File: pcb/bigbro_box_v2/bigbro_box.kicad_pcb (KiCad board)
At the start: 2 copper layers, 100 x 58 mm, 44 parts, among them J1 Current Sense, J2 Display, J3 Mains, J4 Debug, J5 RFID, J6 Relay, J7 Ext, K1 G5LE-1, Q1 MMBT3904, Q2 MMBT3904, Q3 BSS138, Q4 MMBT3906, SW1 Card switch, U1 ESP32-WROOM-32, U2 AP1117-33, U3 4011, U4 4011, U5 RDM6300

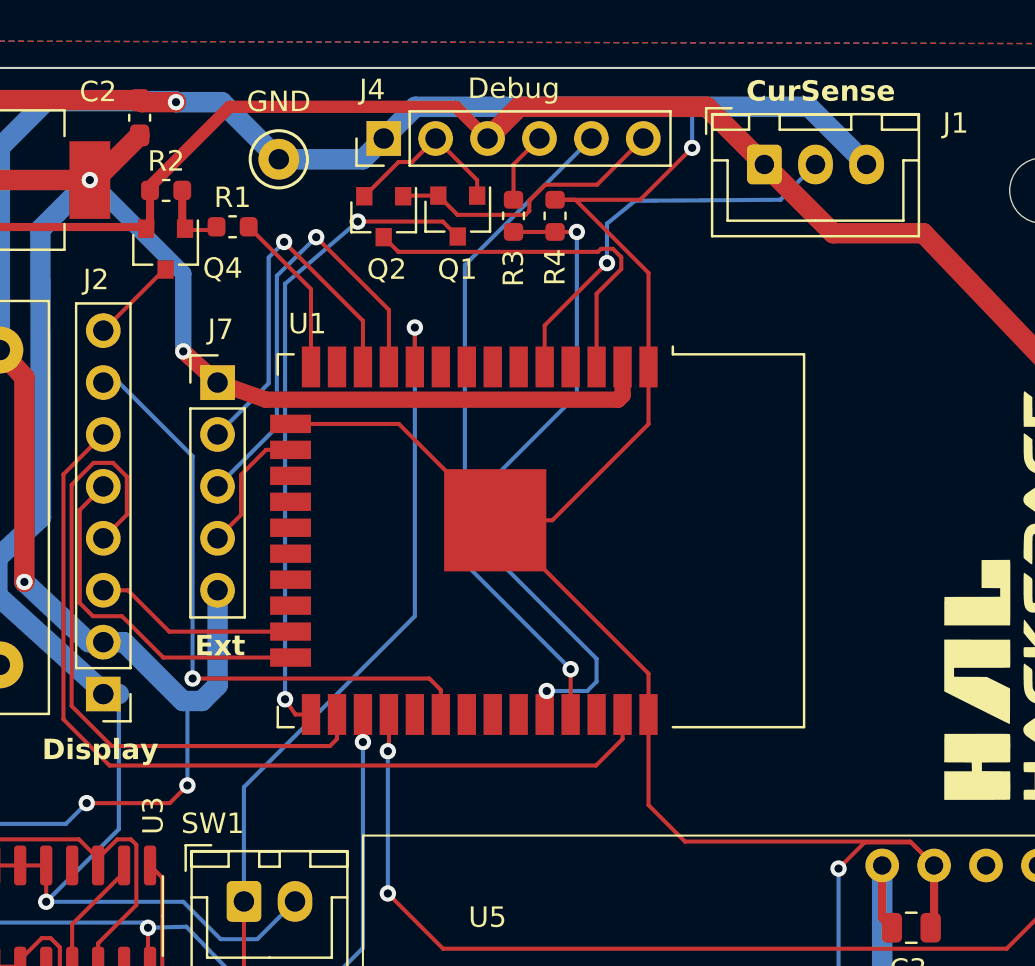
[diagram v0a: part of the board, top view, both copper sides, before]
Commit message: Order.
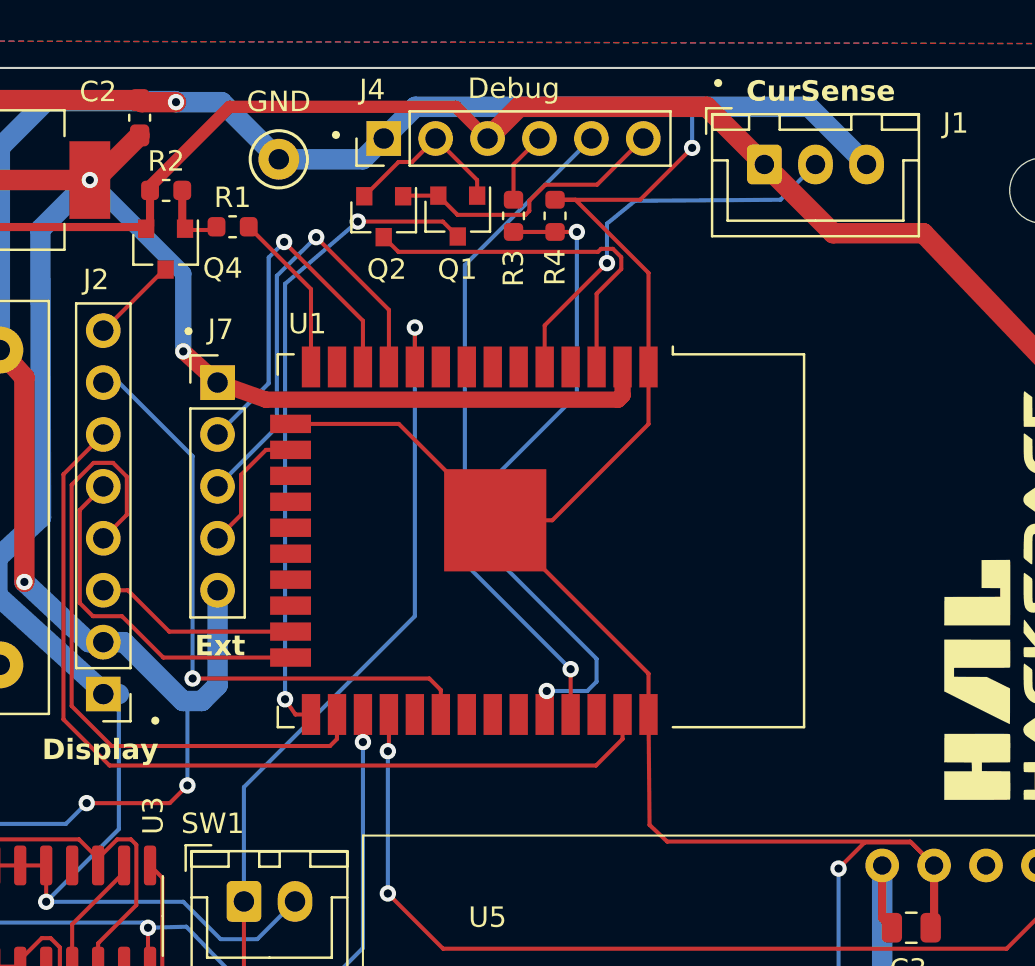
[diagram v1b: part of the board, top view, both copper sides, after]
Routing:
- net GND: track 282.3 -> 282.8 mm
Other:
- board text added: "•"
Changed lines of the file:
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@@
     (pad "1" thru_hole circle (at 0 0) (size 2 2) (drill 1) (layers "*.Cu" "*.Mask")
       (net 2 "GND") (pinfunction "1") (pintype "passive"))
-    (model "${KICAD6_3DMODEL_DIR}/TestPoint.3dshapes/TestPoint_Keystone_5000-5004_Miniature.wrl"
+    (model "${KIPRJMOD}/lib/3D/TestPoint_Loop_D2.60mm_Drill0.9mm_Beaded.step"
       (offset (xyz 0 0 0))
       (scale (xyz 1 1 1))
@@
     (effects (font (size 1 1) (thickness 0.18) bold) (justify left bottom))
   )
+  (gr_text "•" (at 126.8476 60.9092) (layer "F.SilkS")
+    (effects (font (size 1 1) (thickness 0.15)) (justify left bottom mirror))
+  )
   (gr_text "N" (at 67.056 86.36) (layer "F.SilkS")
     (effects (font (size 1.5 1.5) (thickness 0.3)))
@@
     (effects (font (size 1.5 1.5) (thickness 0.3)))
   )
+  (gr_text "•" (at 119.634 70.5104) (layer "F.SilkS")
+    (effects (font (size 1 1) (thickness 0.15)) (justify left bottom mirror))
+  )
+  (gr_text "•" (at 145.542 58.3692) (layer "F.SilkS")
+    (effects (font (size 1 1) (thickness 0.15)) (justify left bottom mirror))
+  )
   (gr_text "Display" (at 112.0648 90.932) (layer "F.SilkS")
     (effects (font (size 1 1) (thickness 0.18) bold) (justify left bottom))
   )
+  (gr_text "•" (at 118.0084 89.5604) (layer "F.SilkS")
+    (effects (font (size 1 1) (thickness 0.15)) (justify left bottom mirror))
+  )
   (gr_text "GND" (at 122.0724 59.2328) (layer "F.SilkS")
     (effects (font (size 1 1) (thickness 0.15)) (justify left bottom))
@@
   (segment (start 153.162 103.632) (end 160.782 111.252) (width 1) (layer "B.Cu") (net 1))
   (segment (start 107.0356 101.4476) (end 107.0356 89.1644) (width 0.2) (layer "B.Cu") (net 1))
-  (segment (start 141.732 88.628) (end 141.732 93.061822) (width 0.2) (layer "F.Cu") (net 2))
   (segment (start 108.204 97.536) (end 108.204 98.806) (width 0.2) (layer "F.Cu") (net 2))
   (segment (start 118.3132 92.964) (end 119.1768 92.1004) (width 0.2) (layer "F.Cu") (net 2))
@@
   (segment (start 112.938 104.722604) (end 112.938 107.858) (width 0.2) (layer "F.Cu") (net 2))
   (segment (start 137.16 63.449) (end 138.155223 63.449) (width 0.2) (layer "F.Cu") (net 2))
-  (segment (start 154.5336 94.8436) (end 155.702 96.012) (width 0.2) (layer "F.Cu") (net 2))
   (segment (start 106.2735 60.184) (end 108.102 60.184) (width 1) (layer "F.Cu") (net 2))
   (segment (start 129.517 74.413) (end 134.232 79.128) (width 0.2) (layer "F.Cu") (net 2))
   (segment (start 124.222 74.413) (end 129.517 74.413) (width 0.2) (layer "F.Cu") (net 2))
-  (segment (start 141.732 93.061822) (end 143.513778 94.8436) (width 0.2) (layer "F.Cu") (net 2))
   (segment (start 108.204 110.701396) (end 109.391604 111.889) (width 0.2) (layer "F.Cu") (net 2))
   (segment (start 109.7125 58.5735) (end 108.102 60.184) (width 1) (layer "F.Cu") (net 2))
@@
   (segment (start 118.618 58.674) (end 116.9405 58.674) (width 1) (layer "F.Cu") (net 2))
   (segment (start 141.3258 63.449) (end 143.8656 60.9092) (width 0.2) (layer "F.Cu") (net 2))
-  (segment (start 143.513778 94.8436) (end 154.5336 94.8436) (width 0.2) (layer "F.Cu") (net 2))
   (segment (start 124.714 103.327) (end 124.765 103.378) (width 0.2) (layer "F.Cu") (net 2))
   (segment (start 111.2012 72.136) (end 110 70.8) (width 1) (layer "F.Cu") (net 2))
   (segment (start 108.204 107.188) (end 108.204 110.701396) (width 0.2) (layer "F.Cu") (net 2))
+  (segment (start 154.5336 94.8436) (end 155.702 96.012) (width 0.2) (layer "F.Cu") (net 2))
   (segment (start 114.808 110.614) (end 116.078 110.614) (width 0.2) (layer "F.Cu") (net 2))
+  (segment (start 141.732 88.628) (end 141.7828 94.0308) (width 0.2) (layer "F.Cu") (net 2))
   (segment (start 111.2012 82.1436) (end 111.2012 72.136) (width 1) (layer "F.Cu") (net 2))
   (segment (start 109.391604 111.889) (end 114.171 111.889) (width 0.2) (layer "F.Cu") (net 2))
@@
   (segment (start 111.557 103.378) (end 111.593396 103.378) (width 0.2) (layer "F.Cu") (net 2))
   (segment (start 107.429 102.121) (end 108.204 101.346) (width 0.2) (layer "F.Cu") (net 2))
+  (segment (start 141.7828 94.0308) (end 142.6464 94.8436) (width 0.2) (layer "F.Cu") (net 2))
+  (segment (start 142.6464 94.8436) (end 154.5336 94.8436) (width 0.2) (layer "F.Cu") (net 2))
   (segment (start 107.2135 93.98) (end 108.204 93.98) (width 0.2) (layer "F.Cu") (net 2))
   (segment (start 116.078 110.614) (end 117.348 110.614) (width 0.2) (layer "F.Cu") (net 2))
@@
       (pts
         (xy 154.7876 94.476)
-        (xy 143.2876 94.476)
-        (xy 143.3892 65.786)
+        (xy 142.932 94.4252)
+        (xy 143.0336 65.7352)
         (xy 154.8892 65.786)
       )
